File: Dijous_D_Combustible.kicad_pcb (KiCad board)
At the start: 2 copper layers, 87.6 x 72.4 mm, 66 parts, among them J1 Screw_Terminal_01x02, J2 Conn_01x02, J3 Conn_02x03_Counter_Clockwise, J4 DE9_Plug, J5 Conn_01x02, J6 Conn_01x02, J7 Conn_01x02, J8 Conn_01x04, K1 Fujitsu_FTR-LYAA005x, K2 Fujitsu_FTR-LYAA005x, Q1 2SC4213, Q2 2SC4213, SW1 SW_Push, U1 MCP2551-I-SN, U2 LM2596S-ADJ, U3 PIC18F258-I/SO, U4 LM1117DT-5.0, U5 MCP4725xxx-xCH, Y1 HC-49-US

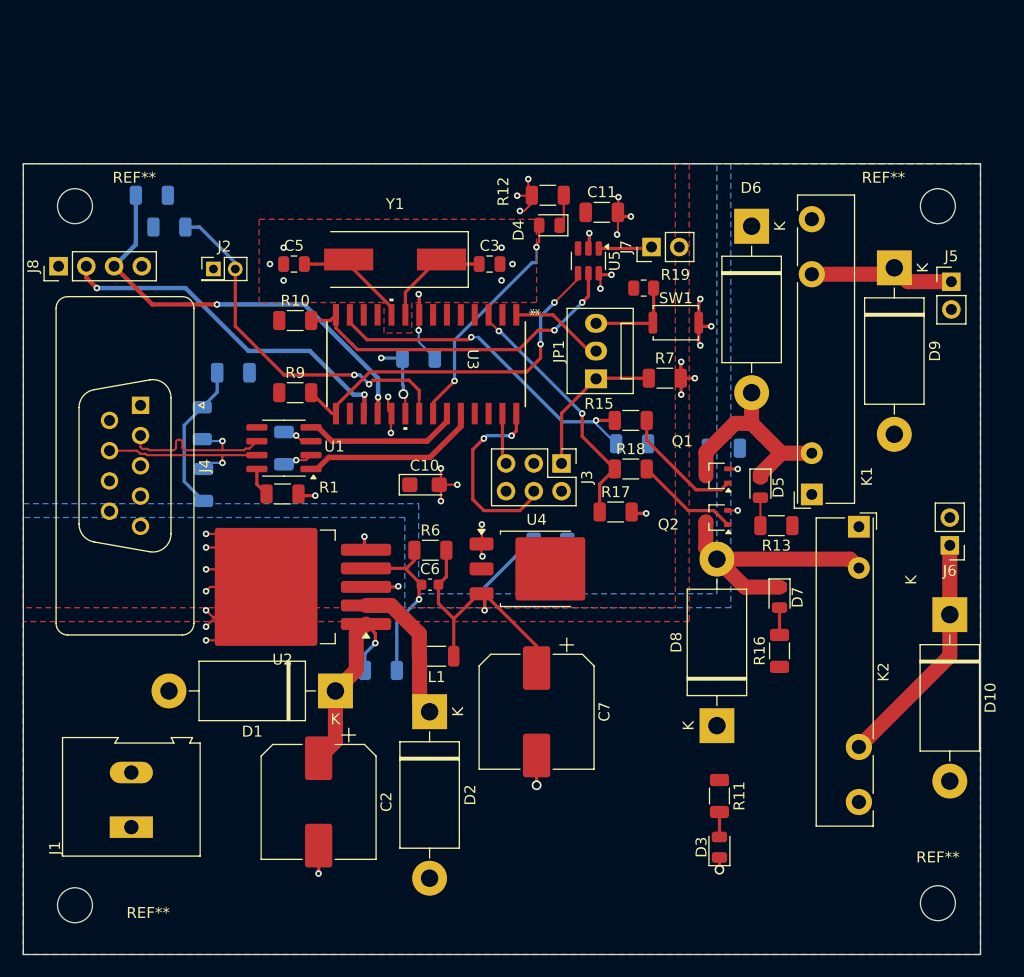
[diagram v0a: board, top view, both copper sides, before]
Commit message: Layout
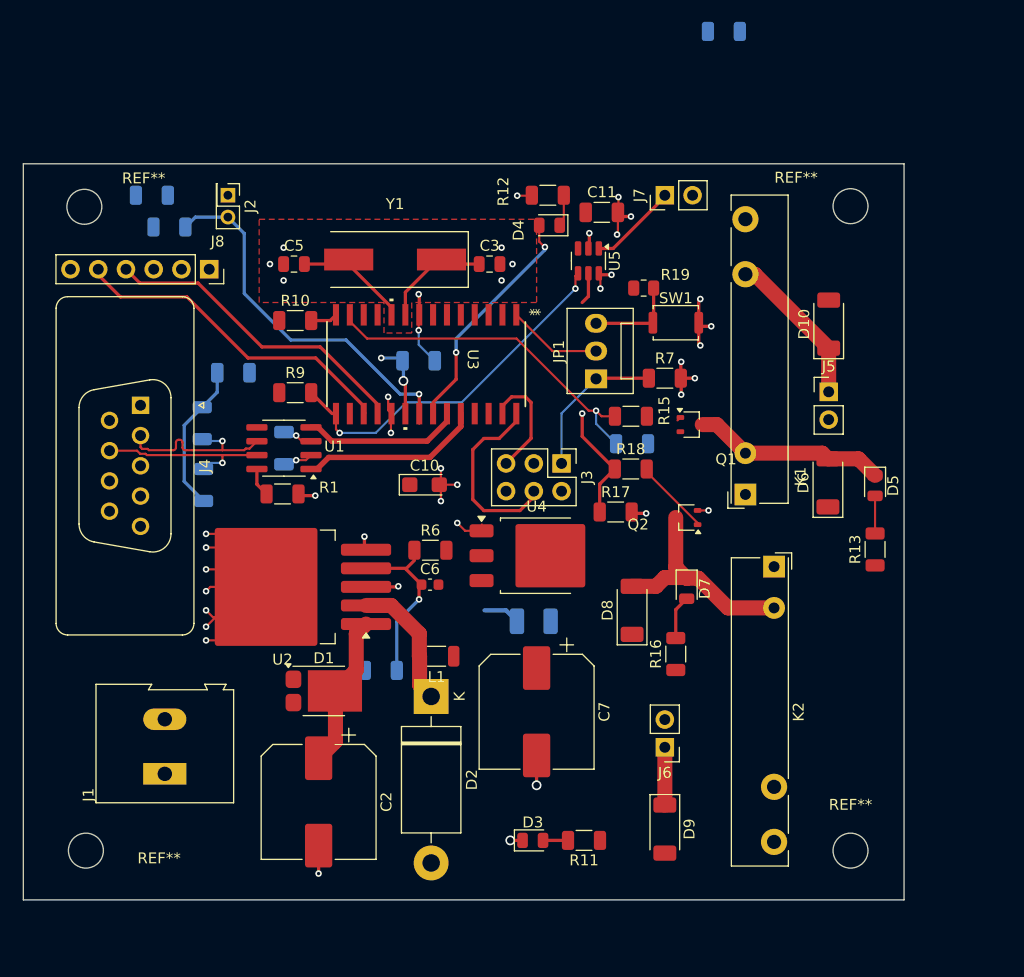
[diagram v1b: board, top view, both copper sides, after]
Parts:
- D1: value MBR340 -> PMEG040V050EPD; footprint Diode_THT:D_DO-201AD_P15.24mm_Horizontal -> Package_TO_SOT_SMD:Nexperia_CFP15_SOT-1289
- D10, D6, D8, D9: value 1N5408 -> PMEG6030EP; footprint Diode_THT:D_DO-201AD_P15.24mm_Horizontal -> Diode_SMD:D_SOD-128
- J8: value Conn_01x04 -> Conn_01x06; footprint Connector_PinHeader_2.54mm:PinHeader_1x04_P2.54mm_Vertical -> Connector_PinSocket_2.54mm:PinSocket_1x06_P2.54mm_Vertical
- moved D9 55.5 mm to (187.0, 132.0)
- moved R4 38.2 mm to (192.4, 59.0)
- moved J6 32.0 mm to (187.0, 124.5)
- moved D10 28.8 mm to (202.0, 85.8), turned to 90 degrees
- moved D6 24.5 mm to (201.9, 100.3), turned to 90 degrees
- moved D3 17.1 mm to (174.9, 133.1), turned to 0 degrees
- moved J5 15.1 mm to (202.0, 92.0)
- moved J8 13.8 mm to (145.3, 80.8), turned to -90 degrees
- moved D8 13.1 mm to (184.0, 112.0)
- moved R11 13.0 mm to (179.6, 133.1), turned to 180 degrees
- moved D5 10.5 mm to (206.2, 100.6)
- moved R16 9.50 mm to (188.0, 116.0)
- moved REF** 9.34 mm to (204.0, 134.0)
- moved R13 9.29 mm to (206.2, 106.4), turned to 90 degrees
- moved K2 8.58 mm to (197.0, 108.0)
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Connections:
- D1 pad 1: Vin_Buck -> Vbat
- D10 pad 1: Solenoide -> Bomba_combustible
- D9 pad 1: Bomba_combustible -> Solenoide
- J8 pad 2: RXD -> unconnected-(J8-Pin_2-Pad2)
- J8 pad 3: TXD -> +5V
- J8 pad 4: +5V -> TXD
- R5 pad 2: GND -> GNDPWR
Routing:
- net Vin_LDO: track 32.7 -> 3.38 mm, vias 1 -> 0
- net SCL: track 31.8 -> 5.40 mm, vias 2 -> 0
- net Solenoide: track 21.9 -> 5.29 mm
- net R_Dipòsit: track 23.5 -> 11.4 mm, vias 2 -> 1
- net Net-(Q1-B): track 11.6 -> 0.57 mm
- net TXD: track 39.7 -> 29.8 mm, vias 2 -> 0
- net PGC: track 4.70 -> 10.9 mm
- net Vin_Buck: track 19.1 -> 14.1 mm, vias 1 -> 0
- net GND: track 48.3 -> 44.6 mm, vias 33 -> 30
- net Retorn_dip: track 24.0 -> 20.5 mm
- net Nivell_combustible: track 4.88 -> 8.15 mm
- net Net-(Q2-B): track 9.54 -> 7.02 mm
- net Retorn_sol: track 19.9 -> 17.7 mm
- net RXD: track 33.4 -> 31.3 mm, vias 2 -> 0
- net Net-(D7-A): track 2.50 -> 4.01 mm
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- removed copper zone on F.Cu, net +5V
- removed copper zone on B.Cu, net GND
- removed copper zone on B.Cu, net GNDPWR
- removed copper zone on F.Cu, net Vbat
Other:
- board size 87.6 x 72.4 mm -> 80.6 x 67.4 mm
